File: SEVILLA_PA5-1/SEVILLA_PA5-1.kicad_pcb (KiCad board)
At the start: 2 copper layers, 64.5 x 56.2 mm, 20 parts, among them J1 MOTOR1 SIGNAL, J10 5V OUTPUT, J2 MOTOR1, J3 MOTOR2 SIGNAL, J4 MOTOR2, J5 MOTOR3 SIGNAL, J6 MOTOR3, J7 Barrel_Jack_Switch, J8 11.1 V OUTPUT, J9 5V OUTPUT, U1 L293D, U2 L293D, U3 LM7809_TO220, U4 LM7805_TO220

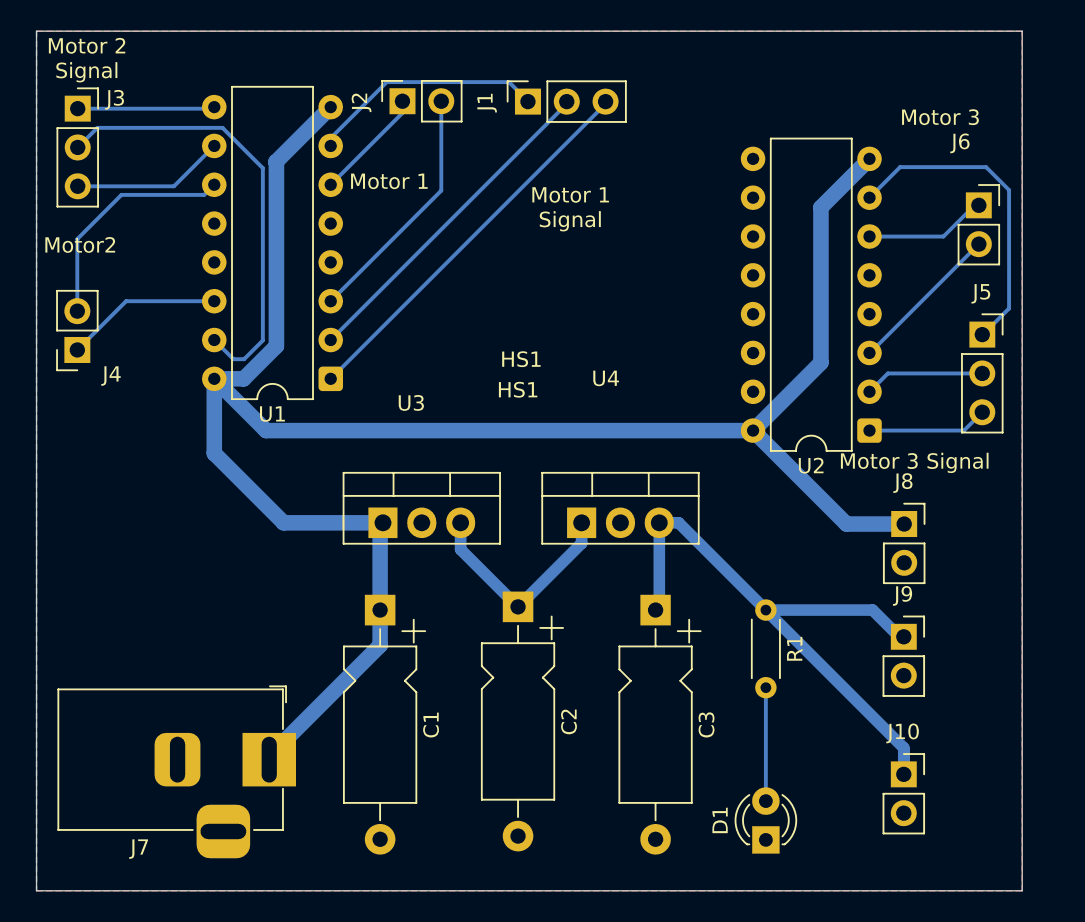
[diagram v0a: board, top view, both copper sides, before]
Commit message: Refactor code structure for improved readability and maintainability
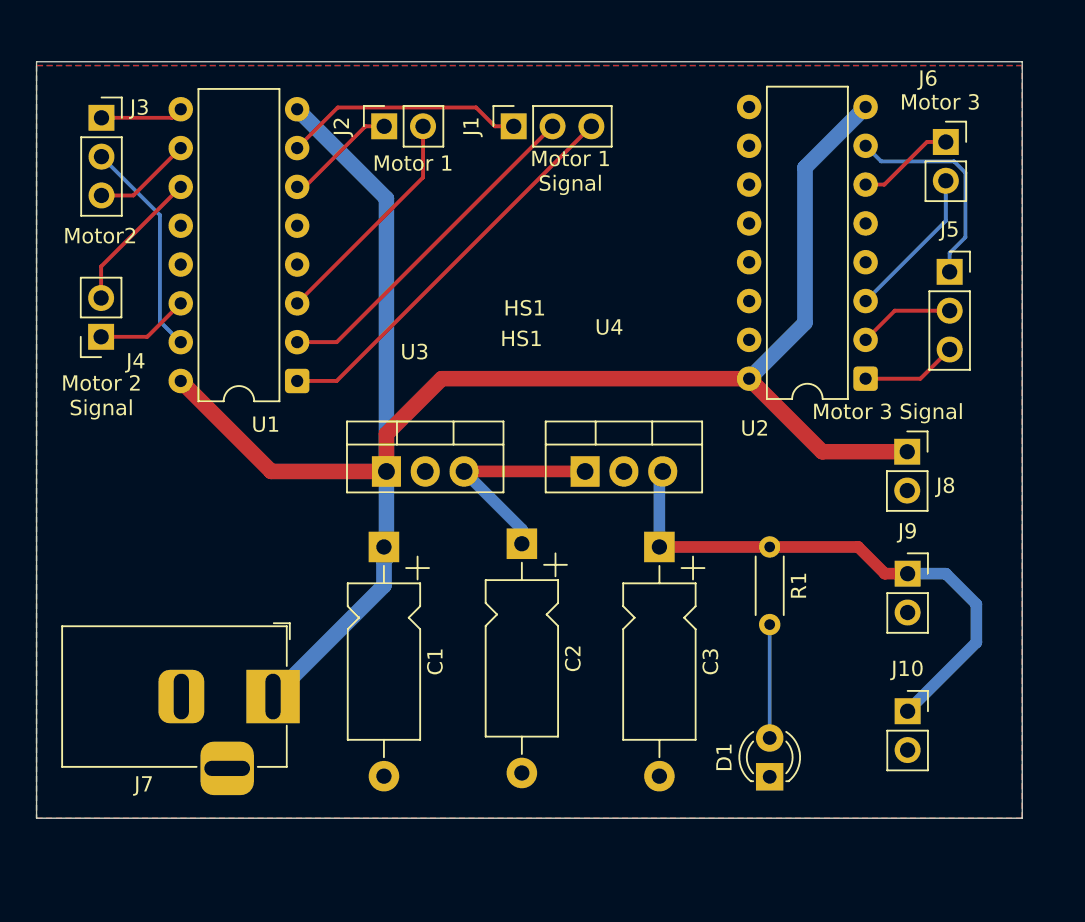
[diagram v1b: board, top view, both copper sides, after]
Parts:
- moved J8 4.73 mm to (157.2, 101.3)
- moved J6 4.68 mm to (159.8, 81.0)
- moved J5 4.63 mm to (160.0, 89.5)
- moved C1 4.14 mm to (123.0, 107.5)
- moved C2 4.14 mm to (132.0, 107.3)
- moved C3 4.14 mm to (141.0, 107.5)
- moved D1 4.14 mm to (148.2, 122.5)
- moved J10 4.14 mm to (157.2, 118.2)
- moved J7 4.14 mm to (115.7, 117.3)
- moved J9 4.14 mm to (157.2, 109.2)
- moved R1 4.14 mm to (148.2, 107.5)
- moved U2 3.41 mm to (154.5, 96.5)
- moved U4 3.37 mm to (136.1, 102.6)
- moved HS1 3.37 mm to (119.0, 106.3)
- moved U3 3.37 mm to (123.1, 102.6)
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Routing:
- net /Motor Driver/FDIRECTION2: track 29.2 -> 14.3 mm
- net /Motor Driver/BDIRECTION3: track 20.8 -> 14.2 mm
- net /Motor Driver/11.1V: track 128.5 -> 122.5 mm
- net /Motor Driver/MOTOR2B: track 15.1 -> 9.43 mm
- net +5V: track 41.1 -> 36.2 mm
- net /Motor Driver/MOTOR2A: track 10.3 -> 6.12 mm
- net /Motor Driver/BDIRECTION2: track 10.0 -> 6.47 mm
- net /Motor Driver/PWM2: track 8.98 -> 5.42 mm
- net /Motor Driver/MOTOR3B: track 8.00 -> 6.41 mm
- net /Motor Driver/PWM3: track 7.88 -> 6.29 mm
- net /Motor Driver/FDIRECTION3: track 7.88 -> 6.29 mm
- net /Motor Driver/MOTOR1A: track 16.1 -> 15.0 mm
- net /Motor Driver/PWM1: track 25.6 -> 26.2 mm
- net /Motor Driver/FDIRECTION1: track 22.0 -> 22.6 mm
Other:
- board size 64.5 x 56.2 mm -> 64.5 x 49.5 mm
